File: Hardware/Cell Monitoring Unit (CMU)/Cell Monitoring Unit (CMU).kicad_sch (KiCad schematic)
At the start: 22 parts, among them J14 JUMPER, J2 LOW SIDE, J4 705550056, J5 HIGH SIDE

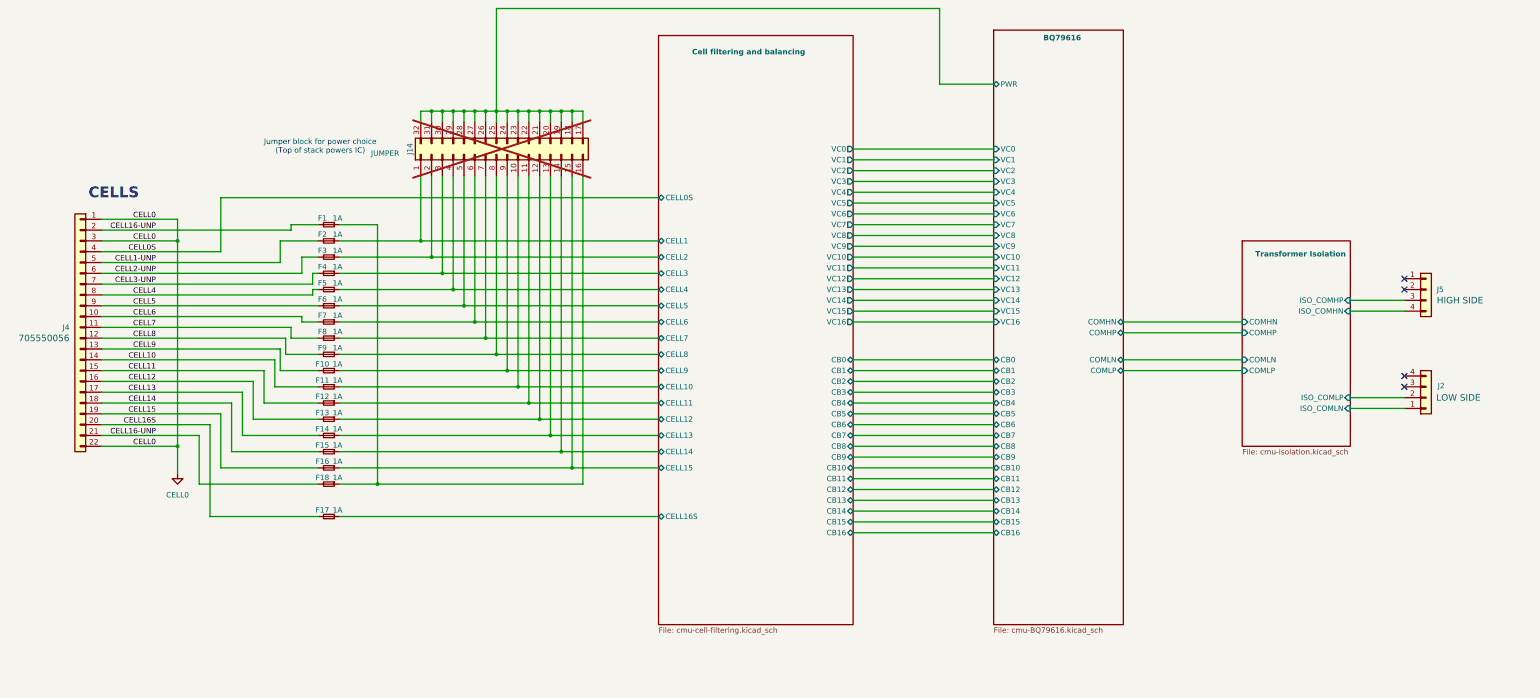
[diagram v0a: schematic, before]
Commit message: updated cmu layout
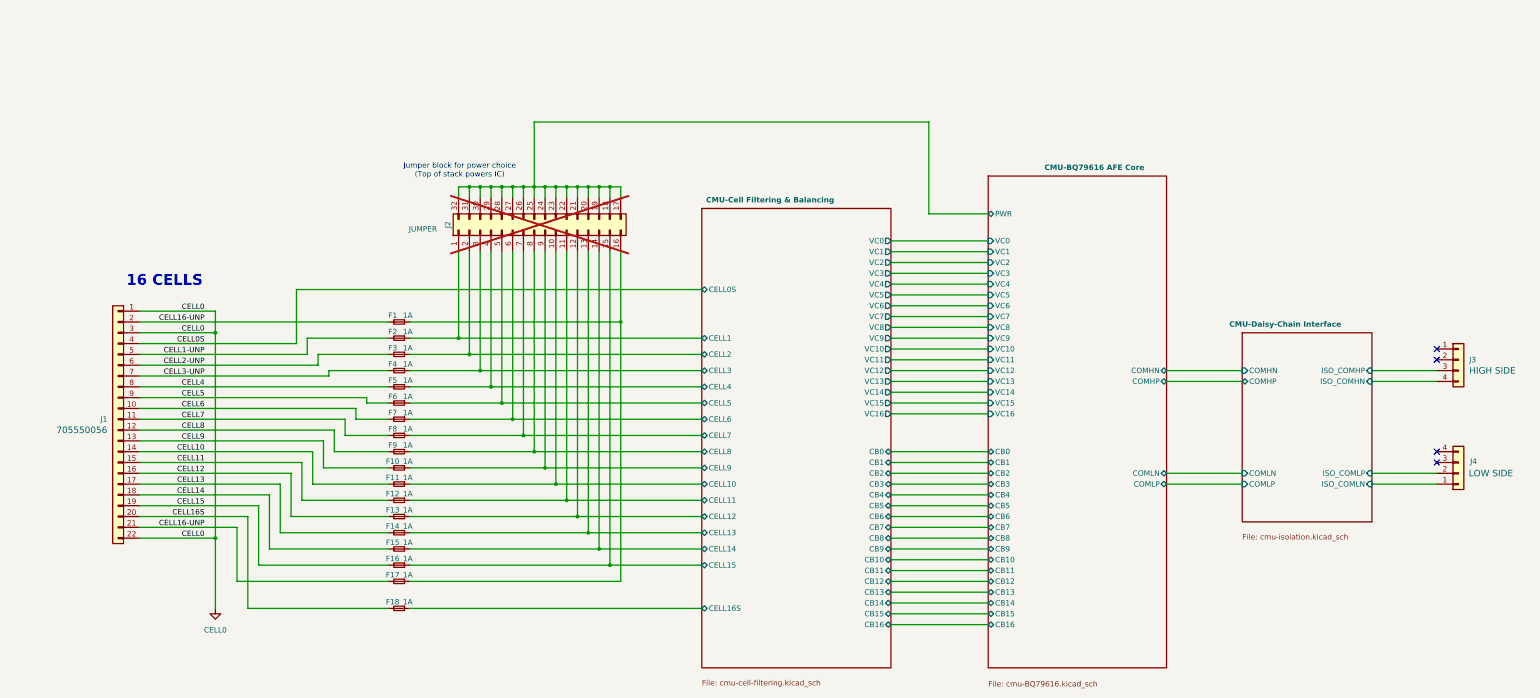
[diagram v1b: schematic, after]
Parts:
- renumbered F18 to F17, F17 to F18, J4 to J1, J14 to J2, J5 to J3, J2 to J4
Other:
- sheet BQ79616 renamed CMU-BQ79616 AFE Core
- sheet Cell filtering and balancing renamed CMU-Cell Filtering & Balancing
- sheet Transformer Isolation renamed CMU-Daisy-Chain Interface
- note added: "16 CELLS"
- note removed: "CELLS"
- moved on the sheet: F1, F10, F11, F12, F13, F14, F15, F16, F17, F18, F2, F3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

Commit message: change iso+update cmu BOM
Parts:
- F1, F10, F11, F12, F13, F14, F15, F16, F17, F18, F2, F3, F4, F5, F6, F7, F8, F9: DIS (none) -> DigiKey; DPN (none) -> 478-F0805B1R00FSCT-ND; MFR (none) -> KYOCERA AVX; MPN (none) -> F0805B1R00FSTR; Purchase Link (none) -> https://www.digikey.com/en/products/detail/kyocera-avx/F080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
- J1: DIS (none) -> Mouser; DPN (none) -> 538-70555-0056; MFR (none) -> Molex; MPN (none) -> 70555-0056; Purchase Link (none) -> https://www.mouser.com/ProductDetail/Molex/70555-0056?qs=RQ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
- J3, J4: DIS (none) -> DigiKey; DPN (none) -> WM14059-ND; MFR (none) -> Molex; MPN (none) -> 705510038; Purchase Link (none) -> https://www.digikey.com/en/products/detail/molex/0705510038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
